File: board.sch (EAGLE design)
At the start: 36 parts, among them K1 RT444012, K2 RT444012, K3 G5LE, Q1 200mA/40V, Q2 200mA/40V, Q3 200mA/40V

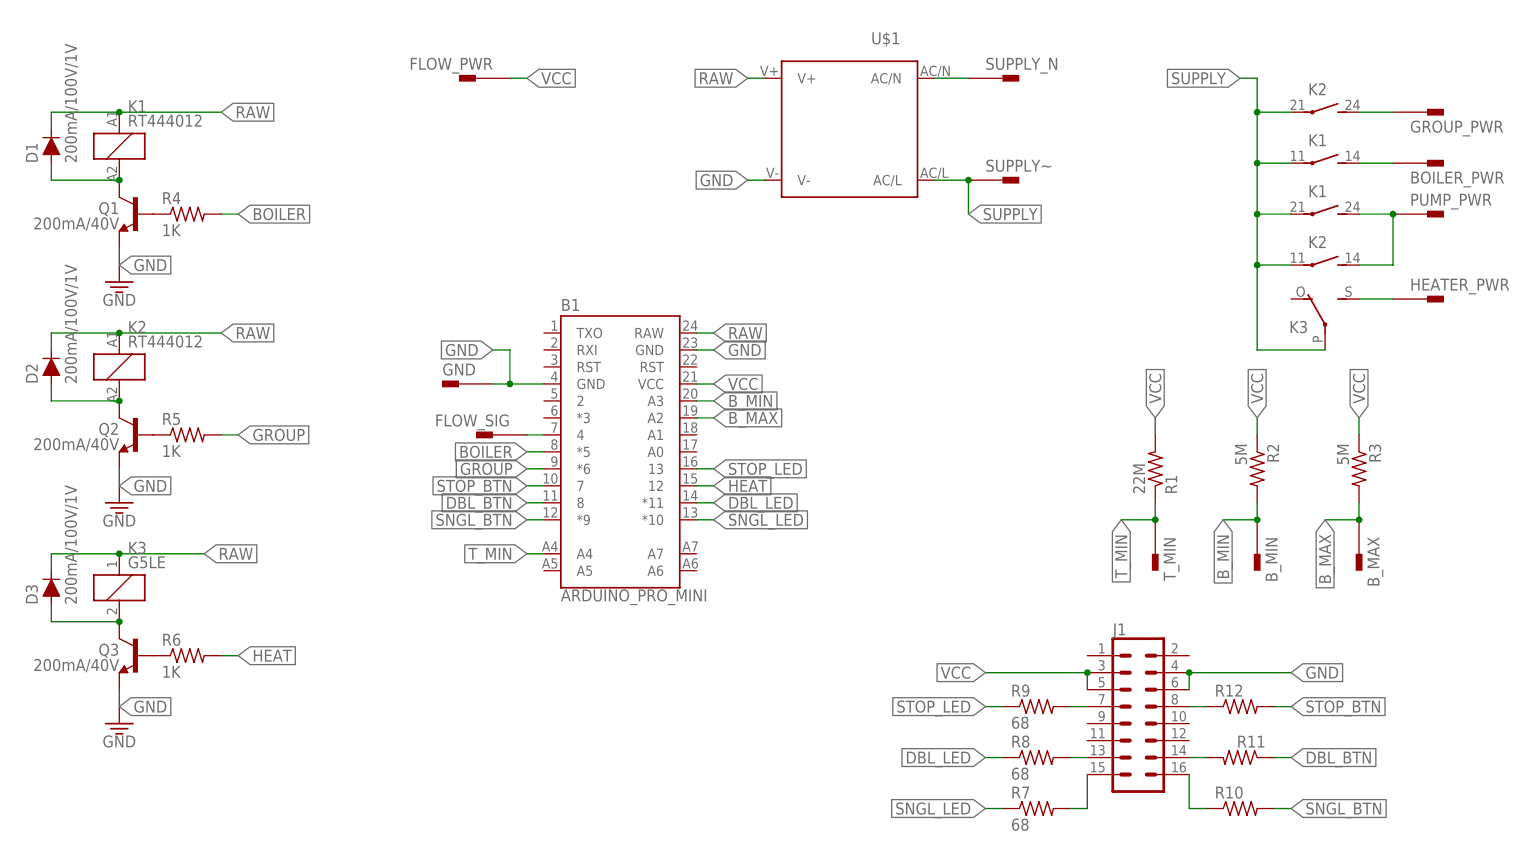
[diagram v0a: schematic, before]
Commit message: did routing. fixed floating buttons. added drill guide?
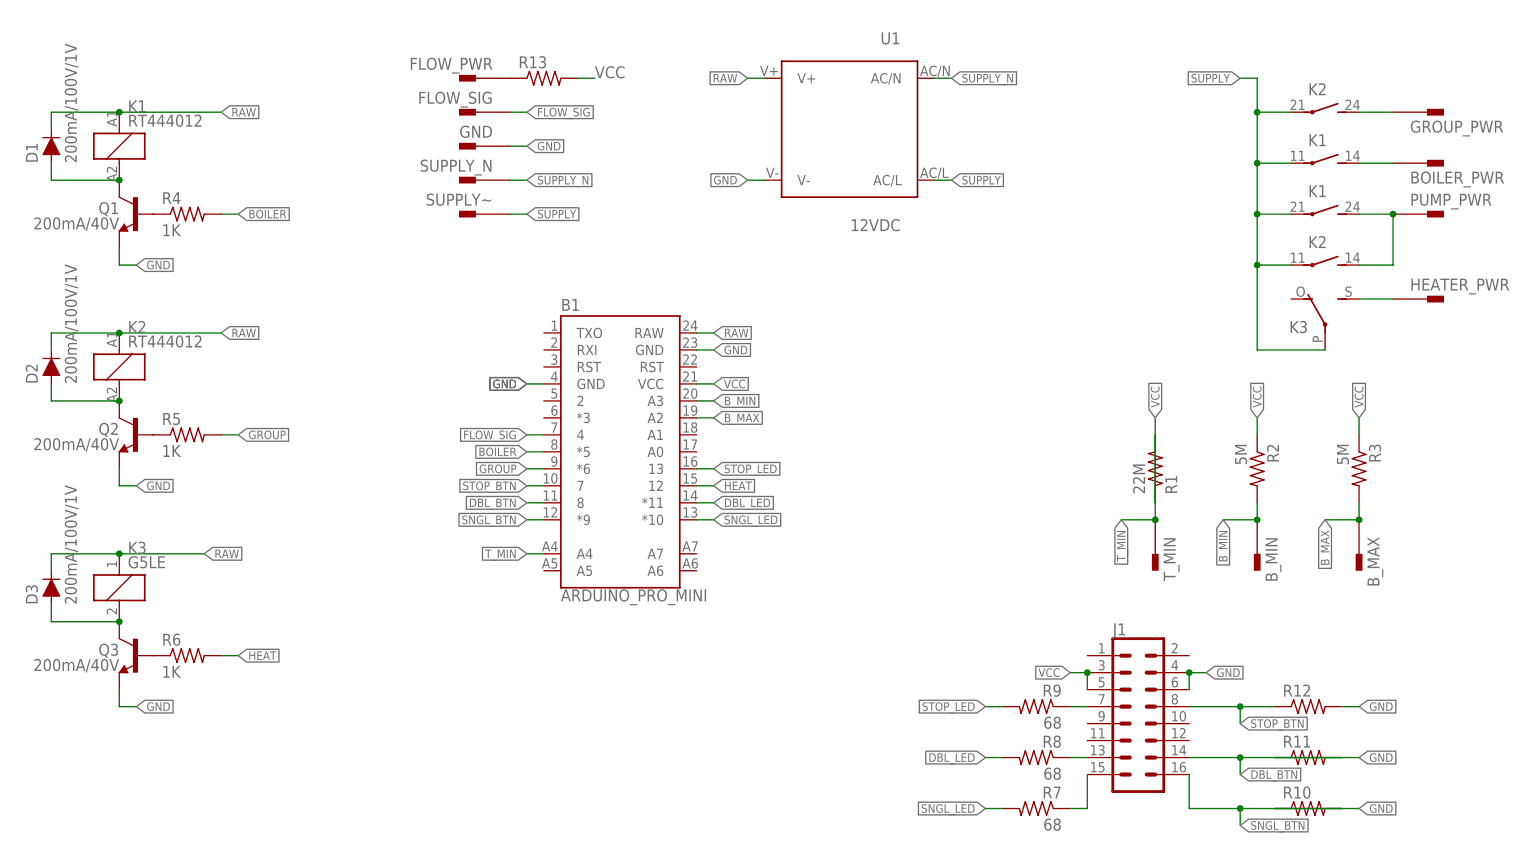
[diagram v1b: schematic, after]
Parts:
- added R13: (no value), rcl:R-US_0207/7
- U1: value (none) -> 12VDC
- renumbered U$1 to U1
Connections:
- net N$3 renamed SUPPLY_N
- net N$8 renamed FLOW_SIG
- removed net N$1: J1.16, R10.1
- removed net N$22: J1.14, R11.2
- removed net N$4: J1.8, R12.1
- new net N$3: FLOW_PWR.1, R13.1
- net DBL_BTN: now also J1.14, R11.2; no longer R11.1
- net DBL_LED: now also R8.2; no longer R8.1
- net GND: now also R10.1, R11.1, R12.2
- net N$14: now also R9.1; no longer R9.2
- net N$23: now also R8.1; no longer R8.2
- net N$24: now also R7.1; no longer R7.2
- net SNGL_BTN: now also J1.16
- net SNGL_LED: now also R7.2; no longer R7.1
- net STOP_BTN: now also J1.8, R12.1; no longer R12.2
- net STOP_LED: now also R9.2; no longer R9.1
- net T_MIN: now also R1.2; no longer R1.1
- net VCC: now also R1.1, R13.2; no longer FLOW_PWR.1, R1.2
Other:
- moved on the sheet: FLOW_SIG, GND, R10, R11, R12, SUPPLY_N, SUPPLY~
